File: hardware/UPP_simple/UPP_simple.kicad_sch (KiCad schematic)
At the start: 9 parts, among them IC2 STM32G0C1KCT6N

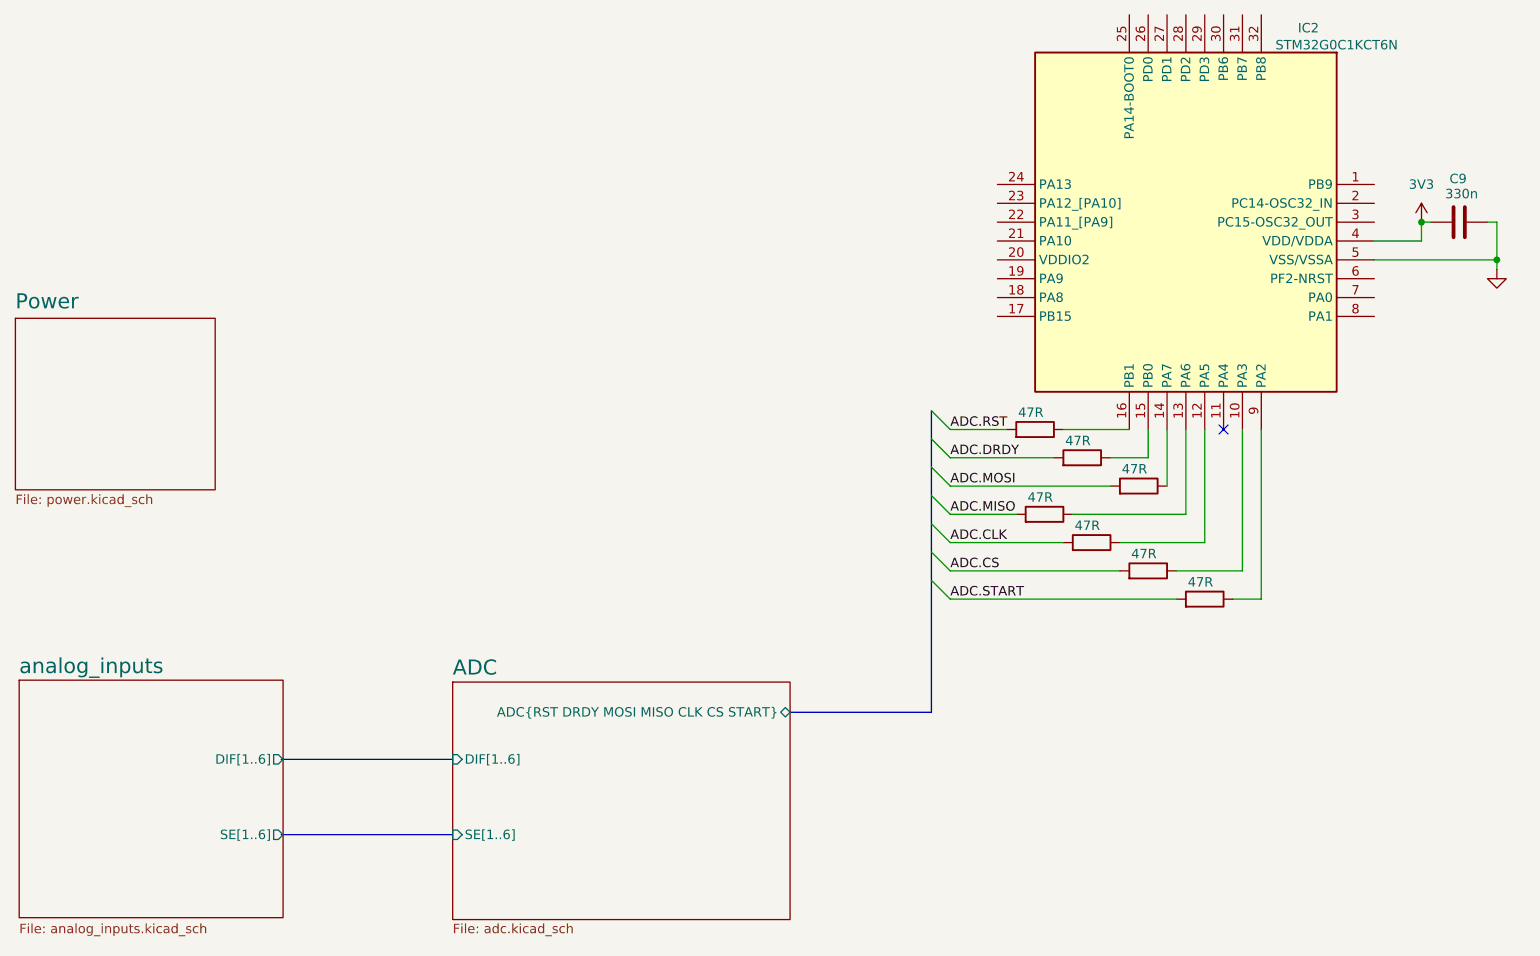
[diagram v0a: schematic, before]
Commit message: Add files via upload
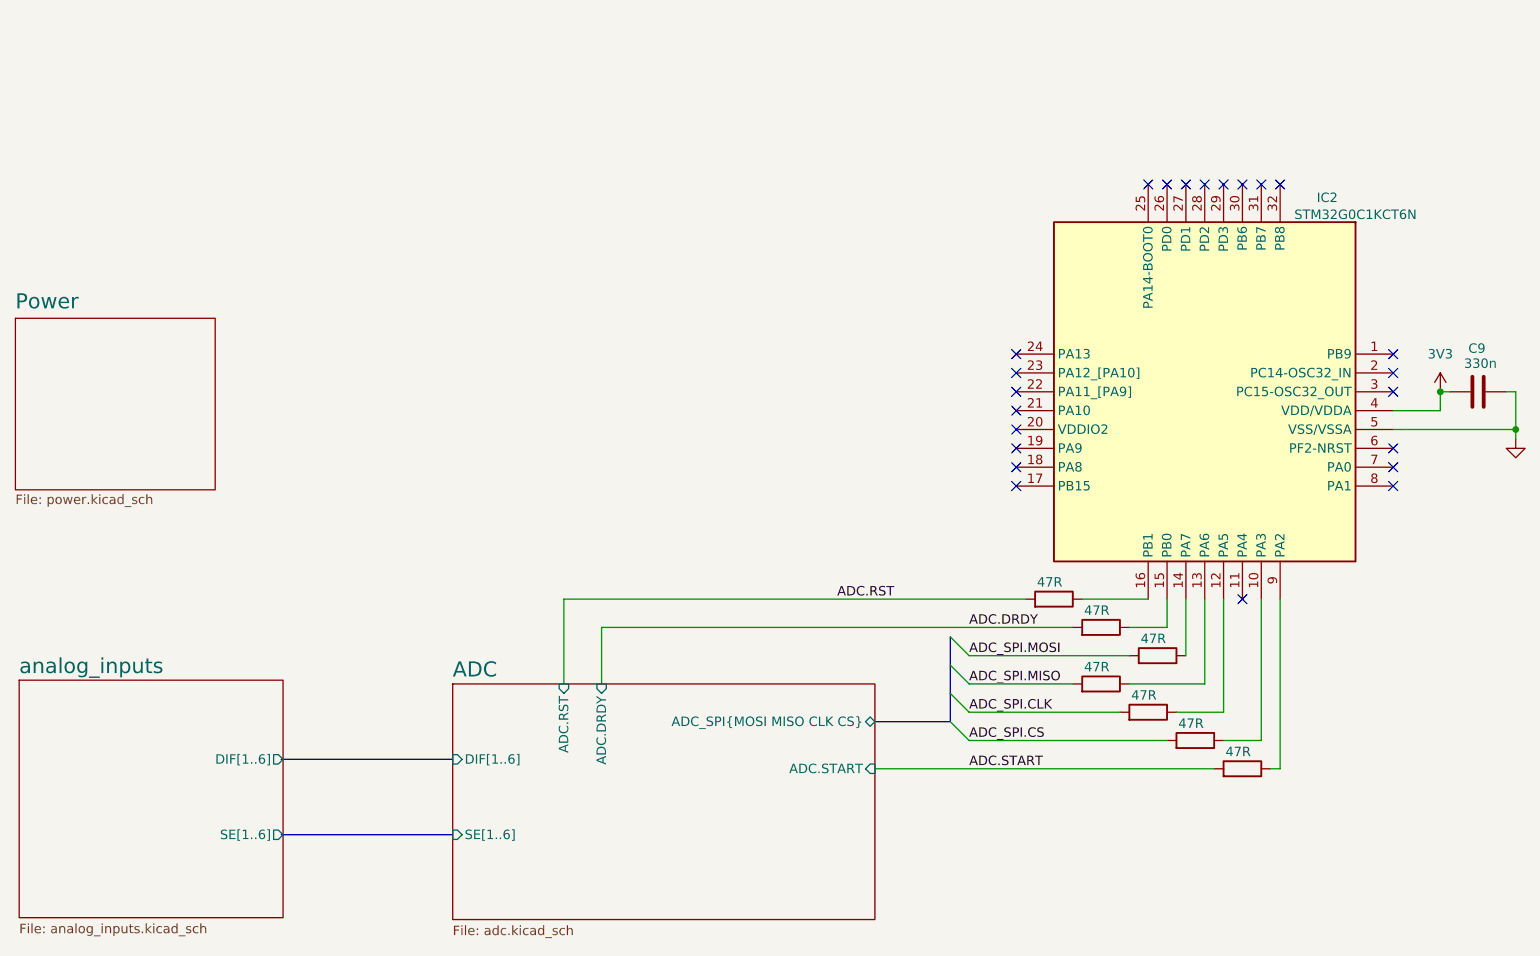
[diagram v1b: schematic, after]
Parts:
- C9: footprint (none) -> Capacitor_SMD:C_0603_1608Metric_Pad1.08x0.95mm_HandSolder
- R10, R11, R12, R13, R14, R15, R9: footprint (none) -> Resistor_SMD:R_0603_1608Metric_Pad0.98x0.95mm_HandSolder
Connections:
- net ADC.MOSI is gone; now on net ADC.DRDY: R9.2
- net ADC.DRDY: no longer R12.2
- net at R9.1: now also IC2.15 (PB0); no longer IC2.14 (PA7)
- net at R12.1: now also IC2.12 (PA5); no longer IC2.15 (PB0)
- net at R11.1: now also IC2.13 (PA6); no longer IC2.12 (PA5)
- net at R10.1: now also IC2.14 (PA7); no longer IC2.13 (PA6)
- net ADC.CLK renamed ADC_SPI.MISO
- net ADC.CS renamed ADC_SPI.CS
- net ADC.MISO renamed ADC_SPI.MOSI
- new net ADC_SPI.CLK: R12.2
- no-connect marks 1 -> 23
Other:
- sheet ADC ports: added ADC.DRDY, ADC.RST, ADC.START, ADC_SPI{MOSI MISO CLK CS}; removed ADC{RST DRDY MOSI MISO CLK CS START}
- moved on the sheet: C9, IC2
